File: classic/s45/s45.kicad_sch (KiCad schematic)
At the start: 96 parts, among them SW1 key, SW10 key, SW11 key, SW12 key, SW13 key, SW14 key, SW15 key, SW16 key, SW17 key, SW18 key, SW19 key, SW2 key, SW20 key, SW21 key, SW22 key, SW23 key, SW24 key, SW25 key, SW26 key, SW27 key, SW28 key, SW29 key, SW3 key, SW30 key, SW31 key, SW32 key, SW33 key, SW34 key, SW35 key, SW36 key, SW37 key, SW38 key, SW39 key, SW4 key, SW40 key, SW41 key, SW42 key, SW43 key, SW44 key, SW45 key, SW5 key, SW6 key, SW7 key, SW8 key, SW9 key, U1 RP2040

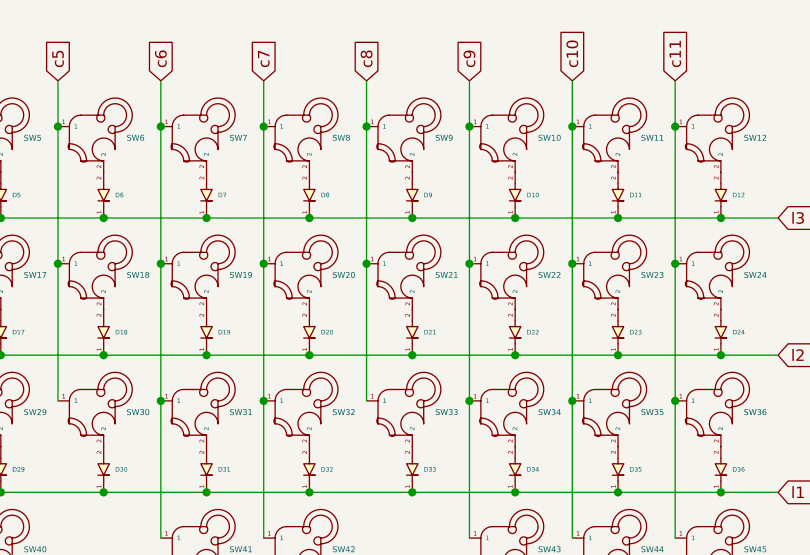
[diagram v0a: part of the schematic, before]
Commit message: sam. 19 oct. 2024 18:38:35 CEST
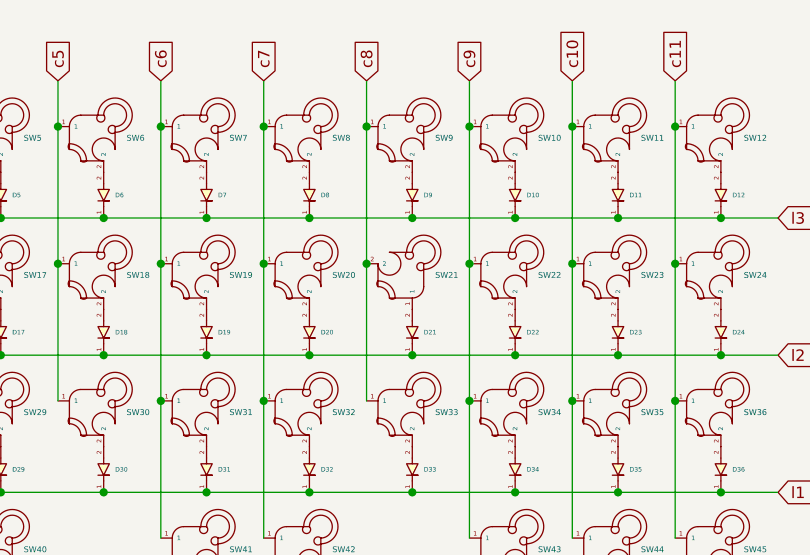
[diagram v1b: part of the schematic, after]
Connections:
- net c8: now also SW21.2; no longer SW21.1
- net at D21.2: now also SW21.1; no longer SW21.2
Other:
- moved on the sheet: SW21
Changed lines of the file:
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@@
 (kicad_sch (version 20211123) (generator eeschema)
   (paper "A4")
+  (junction (at 185.42 105.41) (diameter 0) (color 0 0 0 0)
+  )
+  (junction (at 196.85 105.41) (diameter 0) (color 0 0 0 0)
+  )
+  (junction (at 196.85 59.69) (diameter 0) (color 0 0 0 0)
+  )
+  (junction (at 162.56 74.93) (diameter 0) (color 0 0 0 0)
+  )
+  (junction (at 66.04 49.53) (diameter 0) (color 0 0 0 0)
+  )
+  (junction (at 180.34 49.53) (diameter 0) (color 0 0 0 0)
+  )
+  (junction (at 93.98 74.93) (diameter 0) (color 0 0 0 0)
+  )
+  (junction (at 191.77 80.01) (diameter 0) (color 0 0 0 0)
+  )
+  (junction (at 157.48 49.53) (diameter 0) (color 0 0 0 0)
+  )
+  (junction (at 139.7 90.17) (diameter 0) (color 0 0 0 0)
+  )
   (junction (at 157.48 64.77) (diameter 0) (color 0 0 0 0)
   )
-  (junction (at 185.42 105.41) (diameter 0) (color 0 0 0 0)
-  )
-  (junction (at 196.85 105.41) (diameter 0) (color 0 0 0 0)
-  )
-  (junction (at 196.85 59.69) (diameter 0) (color 0 0 0 0)
-  )
-  (junction (at 162.56 74.93) (diameter 0) (color 0 0 0 0)
-  )
-  (junction (at 66.04 49.53) (diameter 0) (color 0 0 0 0)
-  )
-  (junction (at 180.34 49.53) (diameter 0) (color 0 0 0 0)
-  )
-  (junction (at 93.98 74.93) (diameter 0) (color 0 0 0 0)
-  )
-  (junction (at 191.77 80.01) (diameter 0) (color 0 0 0 0)
-  )
-  (junction (at 157.48 49.53) (diameter 0) (color 0 0 0 0)
-  )
-  (junction (at 139.7 90.17) (diameter 0) (color 0 0 0 0)
-  )
   (junction (at 146.05 64.77) (diameter 0) (color 0 0 0 0)
   )
@@
     (stroke (width 0) (type default) (color 0 0 0 0))
   )
+  (wire (pts (xy 157.48 64.77) (xy 157.48 80.01))
+    (stroke (width 0) (type default) (color 0 0 0 0))
+  )
   (wire (pts (xy 191.77 49.53) (xy 191.77 64.77))
     (stroke (width 0) (type default) (color 0 0 0 0))
@@
   )
   (wire (pts (xy 128.27 59.69) (xy 139.7 59.69))
-    (stroke (width 0) (type default) (color 0 0 0 0))
-  )
-  (wire (pts (xy 157.48 64.77) (xy 157.48 80.01))
     (stroke (width 0) (type default) (color 0 0 0 0))
   )
@@
     (pin "2")
   )
-  (symbol (lib_id "keyb:key") (at 161.29 66.04 0) (unit 1)
-    (in_bom yes) (on_board yes) (fields_autoplaced)
-    (property "Reference" "SW21" (id 0) (at 165.1 66.0399 0)
-      (effects (font (size 0.65 0.65)) (justify left))
-    )
-    (property "Value" "key" (id 1) (at 161.29 62.23 0)
-      (effects (font (size 1.27 1.27)) hide)
-    )
-    (property "Footprint" "keyb-libs:MX-5pin" (id 2) (at 161.29 60.96 0)
-      (effects (font (size 1.27 1.27)) hide)
-    )
+  (symbol (lib_id "keyb:key") (at 161.29 66.04 270) (mirror x) (unit 1)
+    (in_bom yes) (on_board yes) (fields_autoplaced)
+    (property "Reference" "SW21" (id 0) (at 165.1 66.0399 90)
+      (effects (font (size 0.65 0.65)) (justify left))
+    )
+    (property "Value" "key" (id 1) (at 165.1 66.04 0)
+      (effects (font (size 1.27 1.27)) hide)
+    )
+    (property "Footprint" "keyb-libs:MX-5pin" (id 2) (at 166.37 66.04 0)
+      (effects (font (size 1.27 1.27)) hide)
+    )
